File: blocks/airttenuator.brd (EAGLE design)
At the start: 13 x 14.1 mm, 5 parts

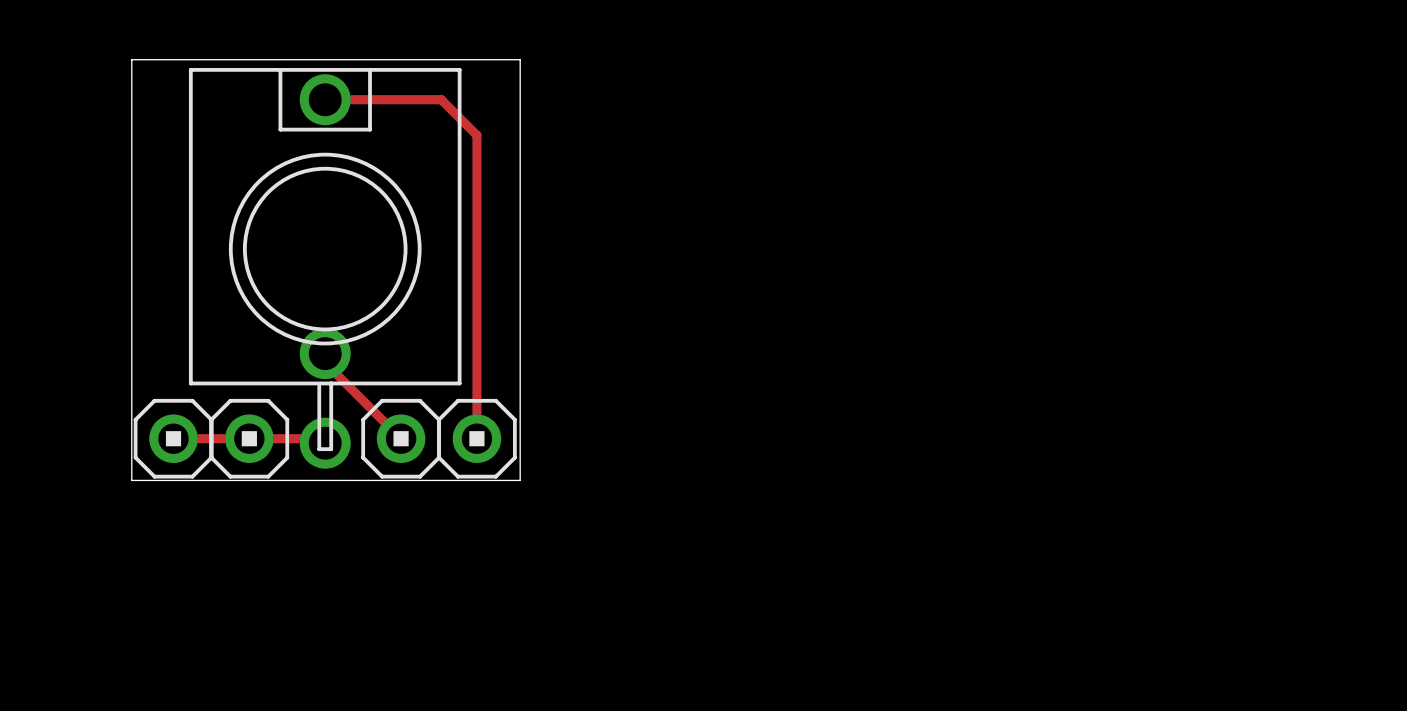
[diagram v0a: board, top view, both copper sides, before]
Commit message: Changes
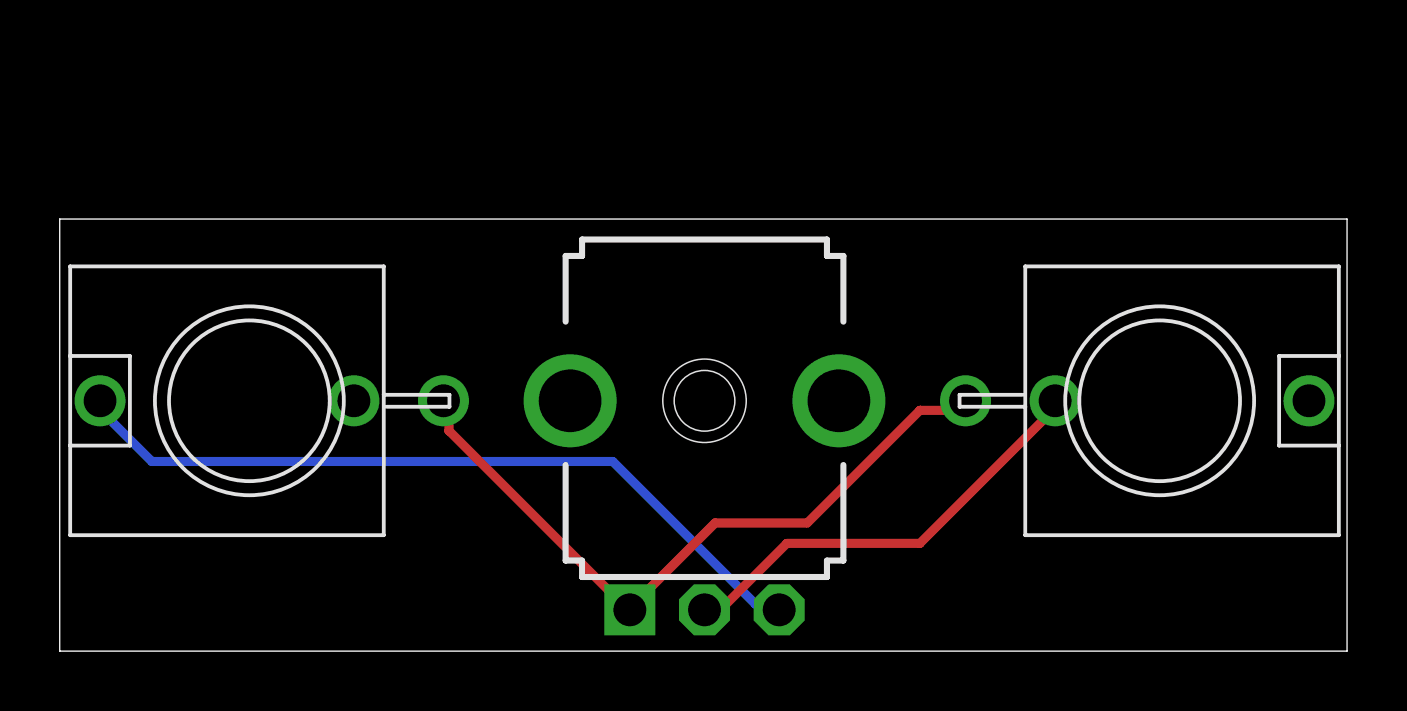
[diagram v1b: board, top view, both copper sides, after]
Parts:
- removed GND, GND1, NORM, SIG: HEADER/MALE/01, connectors:HEADER/MALE/01
- added U$2: WQP-PJ301M-12_JACK, connectors:WQP-PJ301M-12_JACK
- added U$3: (no value), mechanical:PIGATRON-LOGO
- added VR1: 100k, controls:9MM_SNAP-IN_POT
- U$1: device controls:WQP-PJ301M-12_JACK -> connectors:WQP-PJ301M-12_JACK
- moved U$1 28.4 mm to (36.8, 8.89), turned to 270 degrees
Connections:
- removed net N$6: GND.1, GND1.1, U$1.P$3
- new net N$3: U$1.P$2, VR1.2
- net N$1: now also U$1.P$3, U$2.P$3, VR1.1; no longer SIG.1, U$1.P$1
- net N$2: now also U$2.P$1, VR1.3; no longer NORM.1, U$1.P$2
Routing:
- net N$2: track 3.90 -> 25.8 mm
- net N$3: track 0.00 -> 14.8 mm
- net N$1: track 15.7 -> 23.8 mm
- net N$6: track 5.14 -> 0.00 mm
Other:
- board size 13 x 14.1 mm -> 43.1 x 14.5 mm
- board text added: "AIRTTENUATOR"
